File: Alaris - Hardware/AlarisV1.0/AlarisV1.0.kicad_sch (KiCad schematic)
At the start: 5 parts

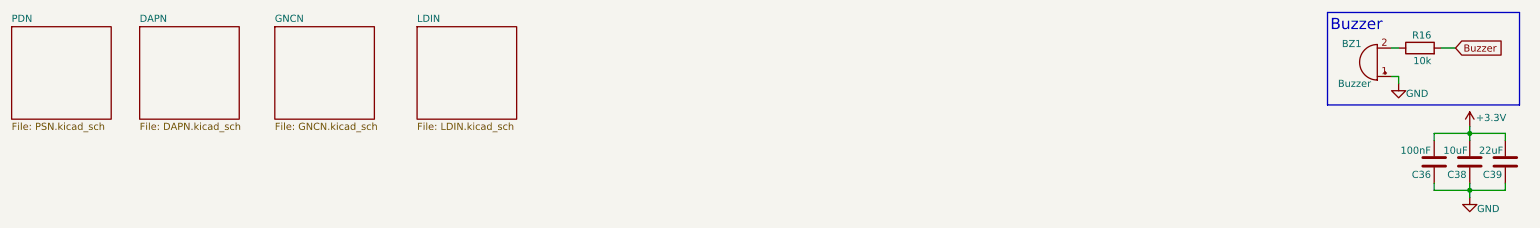
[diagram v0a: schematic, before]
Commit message: Desenvolvimento da PCB
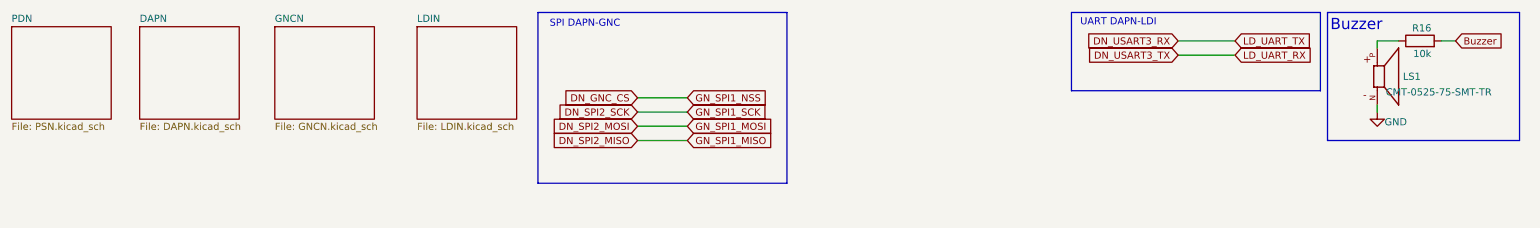
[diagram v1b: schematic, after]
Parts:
- removed BZ1: Buzzer, symbol Device:Buzzer
- removed C36: 100nF, Capacitor_SMD:C_0603_1608Metric_Pad1.08x0.95mm_HandSolder, symbol Device:C
- removed C38: 10uF, Capacitor_SMD:C_0603_1608Metric_Pad1.08x0.95mm_HandSolder, symbol Device:C
- removed C39: 22uF, Capacitor_SMD:C_0603_1608Metric_Pad1.08x0.95mm_HandSolder, symbol Device:C
- added LS1: CMT-0525-75-SMT-TR, Footprint:Buzzer5mm, symbol Buzzer5mm:CMT-0525-75-SMT-TR
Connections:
- net GND: now also LS1.N
- net at R16.1: now also LS1.P
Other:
- note added: "SPI DAPN-GNC"
- note added: "UART DAPN-LDI"
- moved on the sheet: R16
